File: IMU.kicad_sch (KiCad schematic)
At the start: 5 parts, among them U4 BNO085

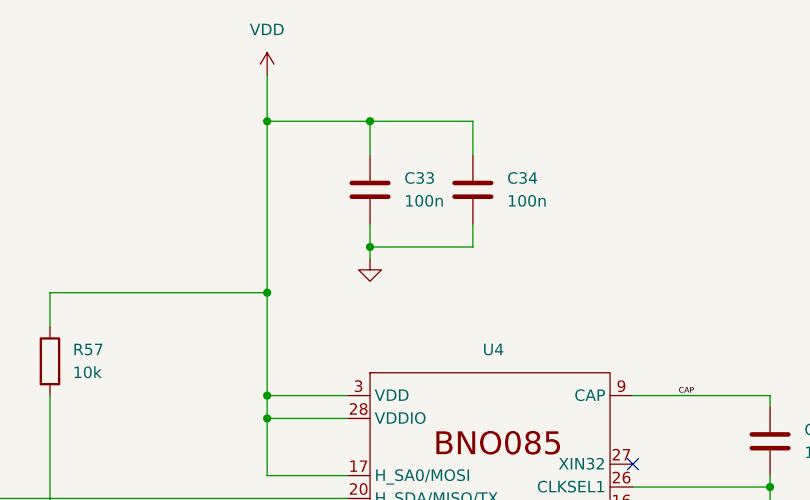
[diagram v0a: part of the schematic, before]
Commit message: Continued routing
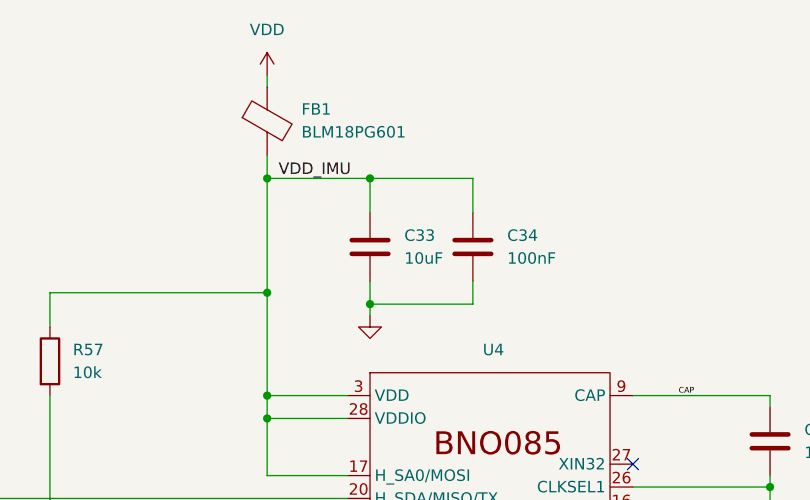
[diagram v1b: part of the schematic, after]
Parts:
- added FB1: BLM18PG601, Inductor_SMD:L_1206_3216Metric, symbol Device:FerriteBead
- C33: value 100n -> 10uF
- C34: value 100n -> 100nF
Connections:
- net VDD: now also FB1.1; no longer C33.1, C34.1, R57.1, U4.17 (H_SA0/MOSI), U4.28 (VDDIO), U4.3 (VDD)
- new net VDD_IMU: C33.1, C34.1, FB1.2, R57.1, U4.17 (H_SA0/MOSI), U4.28 (VDDIO), U4.3 (VDD)
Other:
- moved on the sheet: C33, C34
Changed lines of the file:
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@@
 	)
 	(junction
-		(at 138.43 58.42)
+		(at 138.43 64.77)
 		(diameter 0)
 		(color 0 0 0 0)
@@
 	)
 	(junction
-		(at 138.43 44.45)
+		(at 127 50.8)
+		(diameter 0)
+		(color 0 0 0 0)
+	)
+	(junction
+		(at 138.43 50.8)
 		(diameter 0)
 		(color 0 0 0 0)
@@
 	)
 	(junction
-		(at 127 44.45)
-		(diameter 0)
-		(color 0 0 0 0)
-	)
-	(junction
 		(at 102.87 93.98)
 		(diameter 0)
@@
 	(wire
 		(pts
-			(xy 138.43 48.26) (xy 138.43 44.45)
+			(xy 127 48.26) (xy 127 50.8)
+		)
+		(stroke
+			(width 0)
+			(type default)
+		)
+	)
+	(wire
+		(pts
+			(xy 138.43 54.61) (xy 138.43 50.8)
 		)
 		(stroke
@@
 	(wire
 		(pts
-			(xy 149.86 48.26) (xy 149.86 44.45)
+			(xy 149.86 54.61) (xy 149.86 50.8)
 		)
 		(stroke
@@
 	(wire
 		(pts
-			(xy 149.86 44.45) (xy 138.43 44.45)
+			(xy 149.86 50.8) (xy 138.43 50.8)
 		)
 		(stroke
@@
 	(wire
 		(pts
-			(xy 149.86 58.42) (xy 138.43 58.42)
-		)
-		(stroke
-			(width 0)
-			(type default)
-		)
-	)
-	(wire
-		(pts
-			(xy 149.86 55.88) (xy 149.86 58.42)
-		)
-		(stroke
-			(width 0)
-			(type default)
-		)
-	)
-	(wire
-		(pts
-			(xy 127 39.37) (xy 127 44.45)
+			(xy 149.86 64.77) (xy 138.43 64.77)
+		)
+		(stroke
+			(width 0)
+			(type default)
+		)
+	)
+	(wire
+		(pts
+			(xy 149.86 62.23) (xy 149.86 64.77)
 		)
 		(stroke
@@
 	(wire
 		(pts
+			(xy 127 50.8) (xy 127 63.5)
+		)
+		(stroke
+			(width 0)
+			(type default)
+		)
+	)
+	(wire
+		(pts
 			(xy 128.27 91.44) (xy 135.89 91.44)
 		)
@@
 	(wire
 		(pts
-			(xy 138.43 55.88) (xy 138.43 58.42)
+			(xy 138.43 62.23) (xy 138.43 64.77)
 		)
 		(stroke
@@
 	(wire
 		(pts
-			(xy 127 44.45) (xy 127 63.5)
+			(xy 127 39.37) (xy 127 40.64)
 		)
 		(stroke
@@
 	(wire
 		(pts
-			(xy 138.43 58.42) (xy 138.43 59.69)
-		)
-		(stroke
-			(width 0)
-			(type default)
-		)
-	)
-	(wire
-		(pts
-			(xy 138.43 44.45) (xy 127 44.45)
-		)
-		(stroke
-			(width 0)
-			(type default)
+			(xy 138.43 64.77) (xy 138.43 66.04)
+		)
+		(stroke
+			(width 0)
+			(type default)
+		)
+	)
+	(wire
+		(pts
+			(xy 138.43 50.8) (xy 127 50.8)
+		)
+		(stroke
+			(width 0)
+			(type default)
+		)
+	)
+	(label "VDD_IMU"
+		(at 128.27 50.8 0)
+		(effects
+			(font
+				(size 1.27 1.27)
+			)
+			(justify left bottom)
 		)
 	)
@@
 	(symbol
 		(lib_id "Device:C")
-		(at 138.43 52.07 0)
+		(at 138.43 58.42 0)
 		(unit 1)
 		(exclude_from_sim no)
@@
 		(fields_autoplaced yes)
 		(property "Reference" "C33"
-			(at 142.24 50.7999 0)
+			(at 142.24 57.1499 0)
 			(effects
 				(font
@@
 			)
 		)
-		(property "Value" "100n"
-			(at 142.24 53.3399 0)
+		(property "Value" "10uF"
+			(at 142.24 59.6899 0)
 			(effects
 				(font
@@
 		)
 		(property "Footprint" "Capacitor_SMD:C_1206_3216Metric"
-			(at 139.3952 55.88 0)
+			(at 139.3952 62.23 0)
 			(effects
 				(font
@@
 		)
 		(property "Datasheet" "~"
-			(at 138.43 52.07 0)
+			(at 138.43 58.42 0)
 			(effects
 				(font
@@
 		)
 		(property "Description" "Unpolarized capacitor"
-			(at 138.43 52.07 0)
+			(at 138.43 58.42 0)
 			(effects
 				(font
@@
 	(symbol
 		(lib_id "power:GND")
-		(at 138.43 59.69 0)
+		(at 138.43 66.04 0)
 		(unit 1)
 		(exclude_from_sim no)
@@
 		(fields_autoplaced yes)
 		(property "Reference" "#PWR071"
+			(at 138.43 72.39 0)
+			(effects
+				(font
+					(size 1.27 1.27)
+				)
+				(hide yes)
+			)
+		)
+		(property "Value" "GND"
+			(at 138.43 71.12 0)
+			(effects
+				(font
+					(size 1.27 1.27)
+				)
+				(hide yes)
+			)
+		)
+		(property "Footprint" ""
 			(at 138.43 66.04 0)
 			(effects
@@
 			)
 		)
-		(property "Value" "GND"
-			(at 138.43 64.77 0)
-			(effects
-				(font
-					(size 1.27 1.27)
-				)
-				(hide yes)
-			)
-		)
-		(property "Footprint" ""
-			(at 138.43 59.69 0)
-			(effects
-				(font
-					(size 1.27 1.27)
-				)
-				(hide yes)
-			)
-		)
 		(property "Datasheet" ""
-			(at 138.43 59.69 0)
+			(at 138.43 66.04 0)
 			(effects
 				(font
@@
 		)
 		(property "Description" "Power symbol creates a global label with name \"GND\" , ground"
-			(at 138.43 59.69 0)
+			(at 138.43 66.04 0)
 			(effects
 				(font
@@
 	(symbol
 		(lib_id "Device:C")
-		(at 149.86 52.07 0)
+		(at 149.86 58.42 0)
 		(unit 1)
 		(exclude_from_sim no)
@@
 		(fields_autoplaced yes)
 		(property "Reference" "C34"
-			(at 153.67 50.7999 0)
+			(at 153.67 57.1499 0)
 			(effects
 				(font
@@
 			)
 		)
-		(property "Value" "100n"
-			(at 153.67 53.3399 0)
+		(property "Value" "100nF"
+			(at 153.67 59.6899 0)
 			(effects
 				(font
@@
 		)
 		(property "Footprint" "Capacitor_SMD:C_1206_3216Metric"
-			(at 150.8252 55.88 0)
+			(at 150.8252 62.23 0)
 			(effects
 				(font
@@
 		)
 		(property "Datasheet" "~"
-			(at 149.86 52.07 0)
+			(at 149.86 58.42 0)
 			(effects
 				(font
@@
 		)
 		(property "Description" "Unpolarized capacitor"
-			(at 149.86 52.07 0)
+			(at 149.86 58.42 0)
 			(effects
 				(font
@@
 					(unit 1)
 				)
+			)
+		)
+	)
+	(symbol
+		(lib_id "Device:FerriteBead")
+		(at 127 44.45 0)
+		(unit 1)
+		(exclude_from_sim no)
+		(in_bom yes)
+		(on_board yes)
+		(dnp no)
+		(fields_autoplaced yes)
+		(property "Reference" "FB1"
+			(at 130.81 43.1291 0)
+			(effects
+				(font
+					(size 1.27 1.27)
+				)
+				(justify left)
+			)
+		)
+		(property "Value" "BLM18PG601"
+			(at 130.81 45.6691 0)
+			(effects
+				(font
+					(size 1.27 1.27)
+				)
+				(justify left)
+			)
+		)
+		(property "Footprint" "Inductor_SMD:L_1206_3216Metric"
+			(at 125.222 44.45 90)
+			(effects
+				(font
+					(size 1.27 1.27)
+				)
+				(hide yes)
+			)
+		)
+		(property "Datasheet" "~"
+			(at 127 44.45 0)
+			(effects
+				(font
+					(size 1.27 1.27)
+				)
+				(hide yes)
+			)
+		)
+		(property "Description" "Ferrite bead"
+			(at 127 44.45 0)
+			(effects
+				(font
+					(size 1.27 1.27)
+				)
+				(hide yes)
+			)
+		)
+		(pin "1"
+		)
+		(pin "2"
+		)
+		(instances
+			(project ""
+				(path "/65429680-7d64-40db-aa5f-8b5d6f88b508/69b294a9-6873-479d-9206-157a1ecbcdf8"
+					(reference "FB1")
+					(unit 1)
+				)
